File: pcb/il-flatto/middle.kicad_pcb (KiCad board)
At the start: 2 copper layers, 88.3 x 63.5 mm, 35 parts, among them J103 ISP, J105 JTAG, Q1 12MHz, X102 SD_Card, X103 BAT

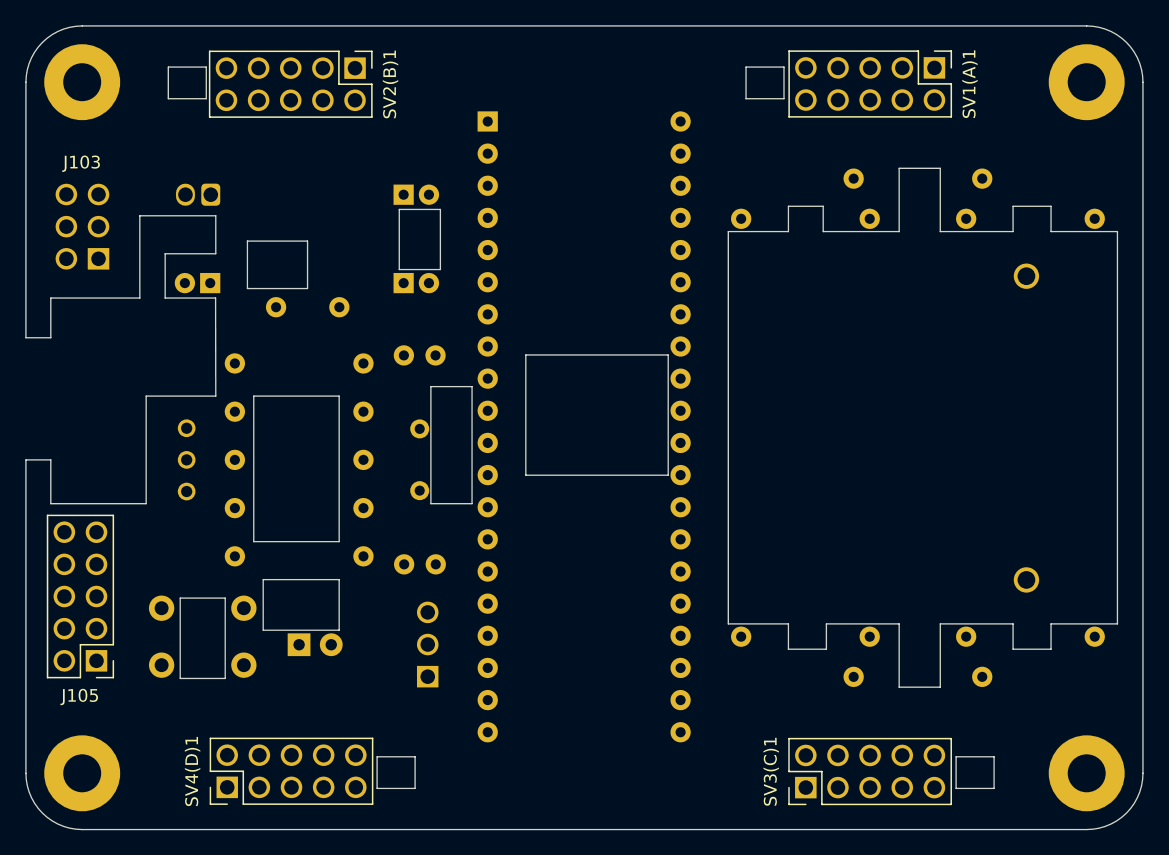
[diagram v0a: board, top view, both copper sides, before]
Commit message: messing around
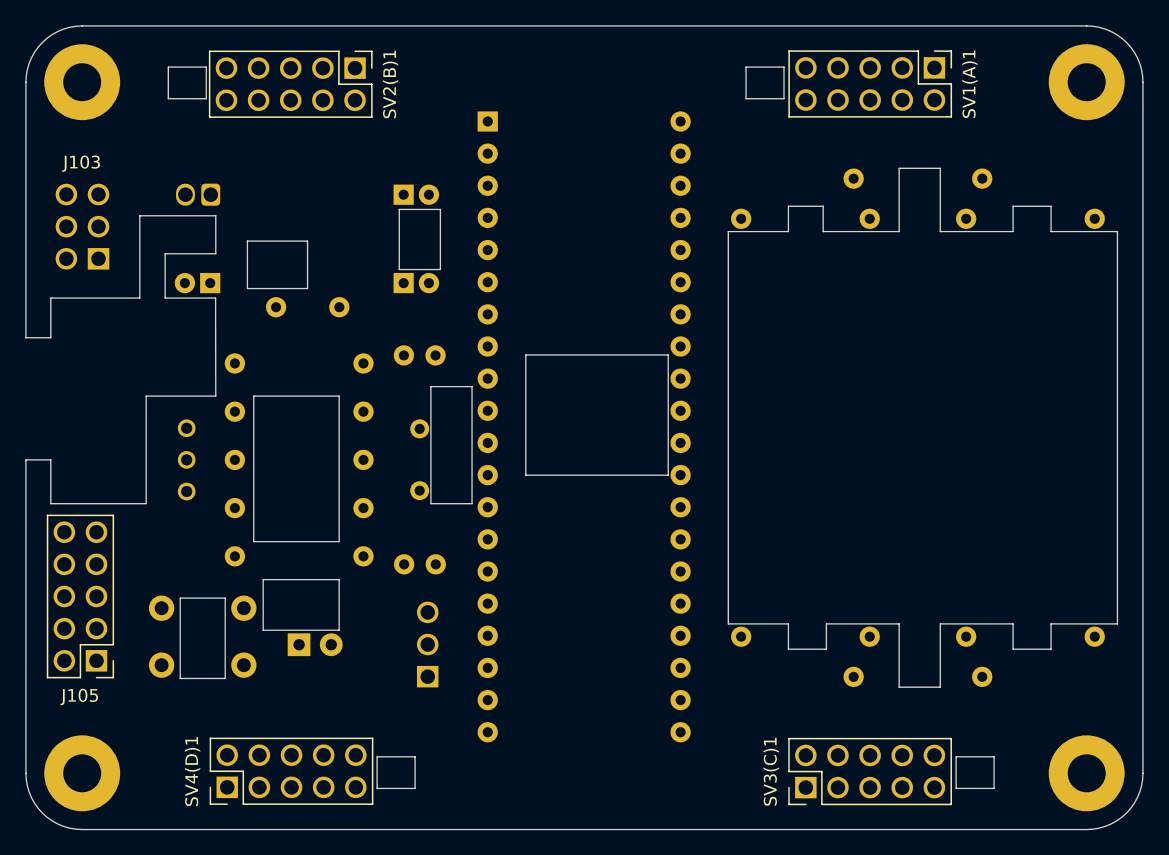
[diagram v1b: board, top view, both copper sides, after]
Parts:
- removed X102: SD_Card, footprints:sd card
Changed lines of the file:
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@@
       (outputformat 1)
       (mirror false)
-      (drillshape 1)
+      (drillshape 0)
       (scaleselection 1)
-      (outputdirectory "")
+      (outputdirectory "output middle/")
     )
   )
@@
       (effects (font (size 1 1) (thickness 0.15)))
     )
-    (pad "1" thru_hole roundrect (at 0 0 180) (size 1.5 1.75) (drill 1.15) (layers F&B.Cu *.Mask) (roundrect_rratio 0.208333)
+    (pad "1" thru_hole roundrect (at 0 0 180) (size 1.5 1.75) (drill 1.15) (layers F&B.Cu *.Mask) (roundrect_rratio 0.2083333333)
       (pinfunction "Pin_1") (pintype "passive"))
     (pad "2" thru_hole oval (at 2 0 180) (size 1.5 1.75) (drill 1.15) (layers F&B.Cu *.Mask)
@@
     )
   )
-  (footprint "footprints:sd card" (layer "F.Cu")
-    (at 166.592079 85.654907 90)
-    (property "Sheetfile" "outer layers.kicad_sch")
-    (property "Sheetname" "externals")
-    (attr board_only exclude_from_pos_files)
-    (fp_text reference "X102" (at 0 -15) (layer "F.SilkS") hide
-      (effects (font (size 1.524 1.524) (thickness 0.3)))
-    )
-    (fp_text value "SD_Card" (at -3.264759 -1.328773 90) (layer "F.SilkS") hide
-      (effects (font (size 1.524 1.524) (thickness 0.3)))
-    )
-    (pad "" thru_hole circle (at -12 0 90) (size 2 2) (drill 1.4) (layers F&B.Cu *.Mask)
-      (zone_connect 2))
-    (pad "" thru_hole circle (at 12 0 90) (size 2 2) (drill 1.4) (layers F&B.Cu *.Mask)
-      (zone_connect 2))
-  )
   (footprint "Package_DIP:DIP-40_W15.24mm" (layer "F.Cu")
